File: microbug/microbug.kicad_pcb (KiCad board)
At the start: 2 copper layers, 31.8 x 38.1 mm, 23 parts, among them J1 Conn_01x03, J2 Conn_01x03, M1 Motor_DC, M2 Motor_DC, U1 ATtiny1616-S, U2 QRE1113GR, U3 TC78H651AFNG, U4 QRE1113GR

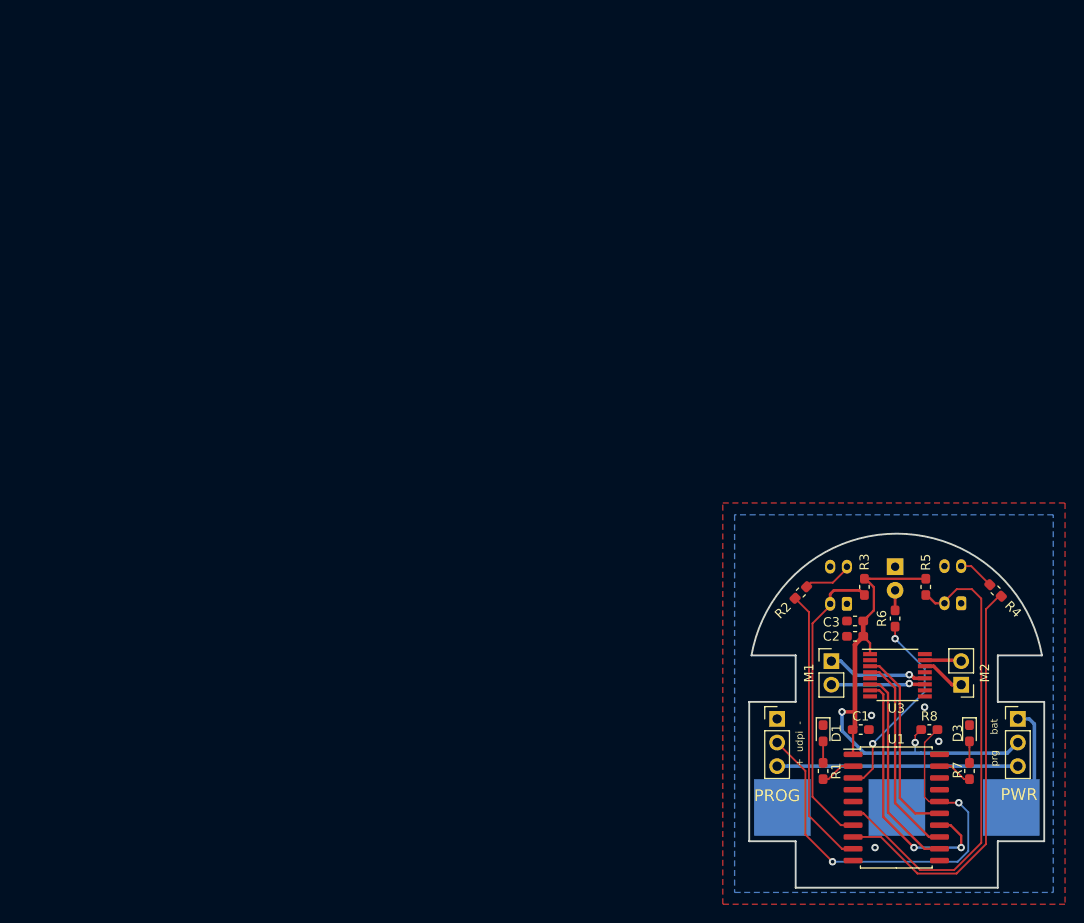
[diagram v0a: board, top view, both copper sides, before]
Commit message: microbug bugging
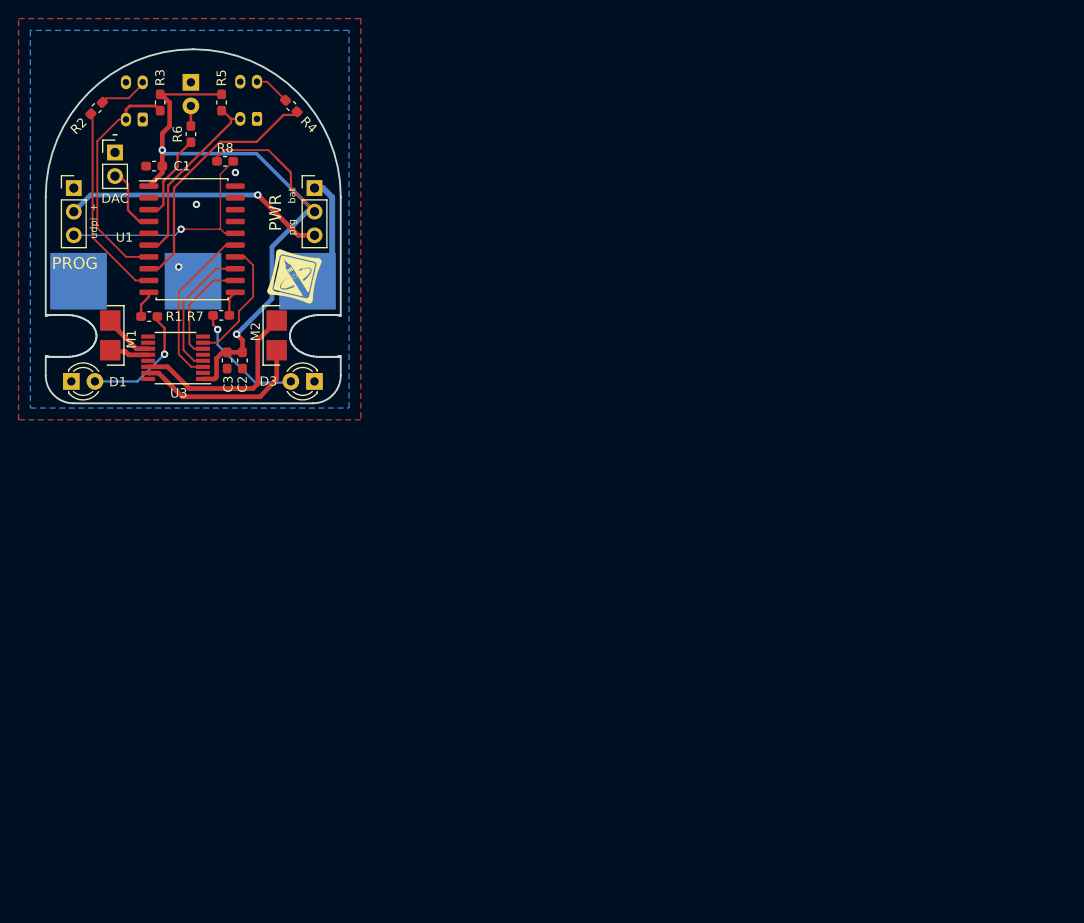
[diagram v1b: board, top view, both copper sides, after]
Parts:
- added G***: LOGO, microbug-fplib:ieee-logo, F.Cu at (85.1, 61.3)
- added J3: Conn_01x02, Connector_PinHeader_2.54mm:PinHeader_1x02_P2.54mm_Vertical, F.Cu at (65.8, 48.0)
- D1, D3: footprint LED_SMD:LED_0603_1608Metric_Pad1.05x0.95mm_HandSolder -> LED_THT:LED_D3.0mm
- M1, M2: footprint Connector_PinHeader_2.54mm:PinHeader_1x02_P2.54mm_Vertical -> microbug-fplib:micro_motor_5mm
- moved U1 97.4 mm to (74.1, 57.3)
- moved R8 97.4 mm to (77.6, 49.0)
- moved C1 97.3 mm to (70.0, 49.5), turned to 180 degrees
- moved J1 94.8 mm to (61.4, 51.8)
- moved J2 94.8 mm to (87.3, 51.8)
- moved BT1 94.6 mm to (74.2, 61.9)
- moved R7 94.3 mm to (77.2, 65.5), turned to 180 degrees
- moved D2 92.0 mm to (74.0, 40.5)
- moved R3 92.0 mm to (70.6, 42.6)
- moved R4 92.0 mm to (84.8, 43.0)
- moved R6 92.0 mm to (74.0, 46.0)
- moved R2 92.0 mm to (63.8, 43.2)
- moved R5 92.0 mm to (77.3, 42.6)
- moved U2 92.0 mm to (68.8, 44.5)
- moved U4 92.0 mm to (81.1, 44.4)
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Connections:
- net Net-(U1-Pad17) renamed /SDA
- net Net-(U1-Pad18) renamed /SCL
- J1 pad 2: /UDPI -> Net-(J1-Pad2)
- J1 pad 3: Net-(J1-Pad3) -> /UDPI
- J2 pad 3: Net-(J1-Pad3) -> Net-(J1-Pad2)
- U1 pad 10: Net-(U1-Pad10) -> /LED1
- U1 pad 11: Net-(U1-Pad11) -> /LED3
- U1 pad 19: /LED3 -> Net-(U1-Pad19)
- U1 pad 2: /LED1 -> Net-(U1-Pad2)
- U1 pad 4: Net-(U1-Pad4) -> /DAC
- U3 pad 11: Net-(M1-Pad2) -> Net-(M1-Pad1)
- U3 pad 12: Net-(M1-Pad1) -> Net-(M1-Pad2)
- U3 pad 14: Net-(M2-Pad1) -> Net-(M2-Pad2)
- U3 pad 15: Net-(M2-Pad2) -> Net-(M2-Pad1)
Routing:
- net /OUT2: track 51.3 -> 20.2 mm
- net Net-(J1-Pad2): track 0.00 -> 28.5 mm, vias 0 -> 1
- net Net-(J1-Pad3): track 25.9 -> 0.00 mm
- net /UDPI: track 47.8 -> 25.7 mm, vias 2 -> 1
- net +3V3: track 56.4 -> 78.0 mm
- net /IR2: track 44.8 -> 27.1 mm
- net Net-(M2-Pad2): track 3.95 -> 20.6 mm
- net /DIR1: track 28.6 -> 13.8 mm, vias 2 -> 0
- net Net-(M2-Pad1): track 4.73 -> 18.8 mm
- net /LED2: track 21.4 -> 9.73 mm, vias 2 -> 0
- net Net-(D1-Pad2): track 2.31 -> 13.1 mm, vias 0 -> 1
- net Net-(D3-Pad2): track 2.31 -> 12.9 mm, vias 0 -> 1
- net /PWM1: track 22.3 -> 13.1 mm
- net /IR1: track 30.2 -> 22.4 mm
- net /DAC: track 0.00 -> 7.53 mm
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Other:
- board size 31.8 x 38.1 mm -> 31.7 x 38.1 mm
- board text added: "-"
- board text added: "DAC"
- board text added: "udpi + -"
- board text removed: "+ udpi -"
